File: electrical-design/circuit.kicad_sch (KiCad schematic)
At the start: 53 parts, among them J1 AVR-ISP-6, Q1 2N3906, Q2 2N3906, Q3 2N3906, Q4 2N3906, SW1 Reset Button, SW2 DS02C-254-1L-04BE, SW3 Reset Button, U1 ATmega8A-P, U2 LTC-4627JR, U3 NE555P, Y1 16MHz

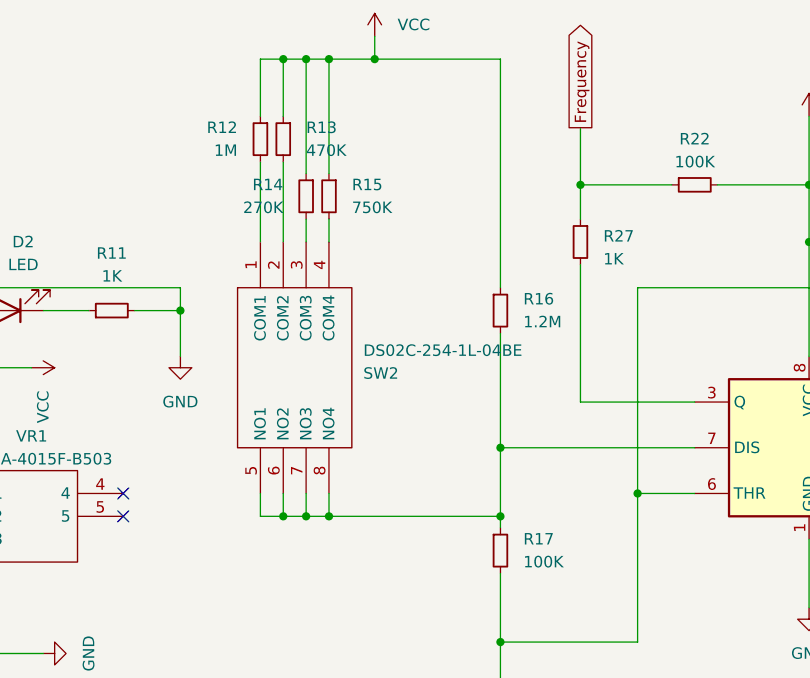
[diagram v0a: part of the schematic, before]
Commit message: Completed Design of 1.2
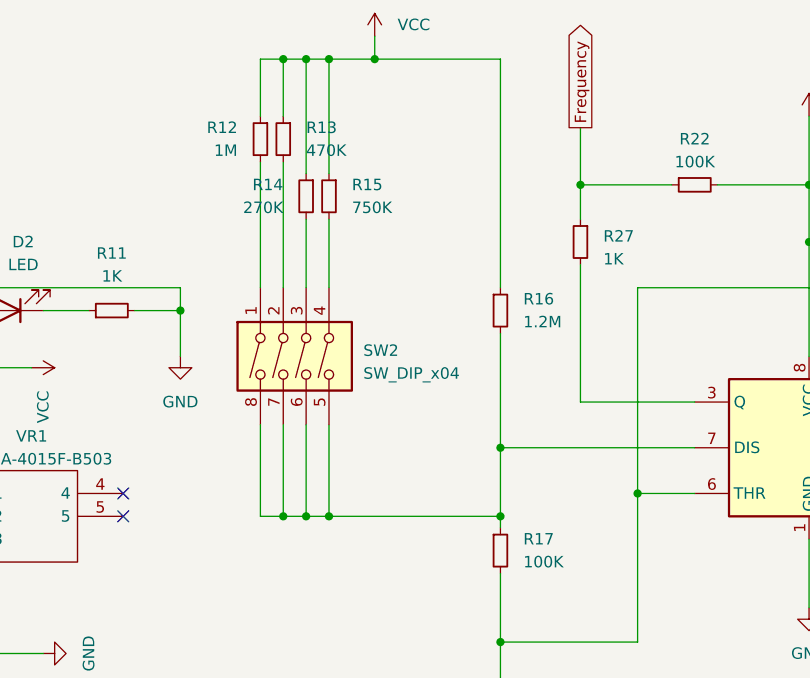
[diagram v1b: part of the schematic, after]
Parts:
- removed SW2: DS02C-254-1L-04BE, DIP Switch:DS02C2541L04BE, symbol DIP Switch:DS02C-254-1L-04BE
- added SW2: SW_DIP_x04, Button_Switch_THT:SW_DIP_SPSTx04_Slide_9.78x12.34mm_W7.62mm_P2.54mm, symbol Switch:SW_DIP_x04
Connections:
- net at R13.2: now also SW2.2
- net at R15.2: now also SW2.4
- net at R12.2: now also SW2.1
- net at R14.2: now also SW2.3
- net at R16.2, R17.1, U3.7 (DIS): now also SW2.5, SW2.6, SW2.7, SW2.8
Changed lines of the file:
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@@
     (stroke (width 0) (type default))
   )
-  (wire (pts (xy 156.21 30.48) (xy 156.21 39.37))
+  (wire (pts (xy 156.21 30.48) (xy 156.21 44.45))
     (stroke (width 0) (type default))
   )
@@
     (stroke (width 0) (type default))
   )
-  (wire (pts (xy 153.67 30.48) (xy 153.67 39.37))
+  (wire (pts (xy 153.67 30.48) (xy 153.67 44.45))
     (stroke (width 0) (type default))
   )
@@
     (stroke (width 0) (type default))
   )
-  (wire (pts (xy 161.29 67.31) (xy 161.29 69.85))
+  (wire (pts (xy 161.29 59.69) (xy 161.29 69.85))
     (stroke (width 0) (type default))
   )
@@
     (stroke (width 0) (type default))
   )
-  (wire (pts (xy 153.67 67.31) (xy 153.67 69.85))
+  (wire (pts (xy 153.67 59.69) (xy 153.67 69.85))
     (stroke (width 0) (type default))
   )
@@
     (stroke (width 0) (type default))
   )
-  (wire (pts (xy 158.75 67.31) (xy 158.75 69.85))
+  (wire (pts (xy 158.75 59.69) (xy 158.75 69.85))
     (stroke (width 0) (type default))
   )
@@
     (stroke (width 0) (type default))
   )
-  (wire (pts (xy 158.75 36.83) (xy 158.75 39.37))
+  (wire (pts (xy 158.75 36.83) (xy 158.75 44.45))
     (stroke (width 0) (type default))
   )
@@
     (stroke (width 0) (type default))
   )
-  (wire (pts (xy 156.21 67.31) (xy 156.21 69.85))
+  (wire (pts (xy 156.21 59.69) (xy 156.21 69.85))
     (stroke (width 0) (type default))
   )
@@
     (stroke (width 0) (type default))
   )
-  (wire (pts (xy 161.29 36.83) (xy 161.29 39.37))
+  (wire (pts (xy 161.29 36.83) (xy 161.29 44.45))
     (stroke (width 0) (type default))
   )
@@
     )
   )
-  (symbol (lib_id "DIP Switch:DS02C-254-1L-04BE") (at 153.67 39.37 90) (mirror x) (unit 1)
-    (in_bom yes) (on_board yes) (dnp no)
-    (property "Reference" "SW2" (at 165.1 53.975 90)
-      (effects (font (size 1.27 1.27)) (justify right))
-    )
-    (property "Value" "DS02C-254-1L-04BE" (at 165.1 51.435 90)
-      (effects (font (size 1.27 1.27)) (justify right))
-    )
-    (property "Footprint" "DIP Switch:DS02C2541L04BE" (at 151.13 63.5 0)
-      (effects (font (size 1.27 1.27)) (justify left) hide)
-    )
-    (property "Datasheet" "https://www.cuidevices.com/product/resource/digikeypdf/ds02-254.pdf" (at 153.67 63.5 0)
-      (effects (font (size 1.27 1.27)) (justify left) hide)
-    )
-    (property "Description" "DIP Switches / SIP Switches DIP Switch, SPST, 2.54 pitch, Raised actuator, convex bottom, long pin, 4 position, Blue" (at 156.21 63.5 0)
-      (effects (font (size 1.27 1.27)) (justify left) hide)
-    )
-    (property "Height" "9.9" (at 158.75 63.5 0)
-      (effects (font (size 1.27 1.27)) (justify left) hide)
-    )
-    (property "Mouser Part Number" "490-DS02C-254-1L04BE" (at 161.29 63.5 0)
-      (effects (font (size 1.27 1.27)) (justify left) hide)
-    )
-    (property "Mouser Price/Stock" "https://www.mouser.co.uk/ProductDetail/CUI-Devices/DS02C-254-1L-04BE?qs=wnTfsH77Xs4EGXqmfKoj6A%3D%3D" (at 163.83 63.5 0)
-      (effects (font (size 1.27 1.27)) (justify left) hide)
-    )
-    (property "Manufacturer_Name" "CUI Devices" (at 166.37 63.5 0)
-      (effects (font (size 1.27 1.27)) (justify left) hide)
-    )
-    (property "Manufacturer_Part_Number" "DS02C-254-1L-04BE" (at 168.91 63.5 0)
-      (effects (font (size 1.27 1.27)) (justify left) hide)
-    )
-    (pin "1")
-    (pin "2")
-    (pin "3")
-    (pin "4")
-    (pin "5")
-    (pin "6")
-    (pin "7")
-    (pin "8")
-    (instances
-      (project "circuit"
-        (path "/e92f8e40-1e47-4cd0-a865-c589067a003b"
-          (reference "SW2") (unit 1)
-        )
-      )
-    )
-  )
   (symbol (lib_id "Device:R_Small") (at 180.34 73.66 0) (unit 1)
     (in_bom yes) (on_board yes) (dnp no) (fields_autoplaced)
@@
         )
       )
+    )
+  )
+  (symbol (lib_id "Switch:SW_DIP_x04") (at 158.75 52.07 90) (mirror x) (unit 1)
+    (in_bom yes) (on_board yes) (dnp no) (fields_autoplaced)
+    (property "Reference" "SW2" (at 165.1 51.435 90)
+      (effects (font (size 1.27 1.27)) (justify right))
+    )
+    (property "Value" "SW_DIP_x04" (at 165.1 53.975 90)
+      (effects (font (size 1.27 1.27)) (justify right))
+    )
+    (property "Footprint" "Button_Switch_THT:SW_DIP_SPSTx04_Slide_9.78x12.34mm_W7.62mm_P2.54mm" (at 158.75 52.07 0)
+      (effects (font (size 1.27 1.27)) hide)
+    )
+    (property "Datasheet" "~" (at 158.75 52.07 0)
+      (effects (font (size 1.27 1.27)) hide)
+    )
+    (pin "1")
+    (pin "2")
+    (pin "3")
+    (pin "4")
+    (pin "5")
+    (pin "6")
+    (pin "7")
+    (pin "8")
+    (instances
+      (project "circuit"
+        (path "/e92f8e40-1e47-4cd0-a865-c589067a003b"
+          (reference "SW2") (unit 1)
+        )
+      )
